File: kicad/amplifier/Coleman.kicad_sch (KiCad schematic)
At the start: 47 parts, among them Q1 TIP122, Q10 TIP122, Q11 IXTP6N50D2, Q12 BC550, Q13 BC550, Q14 TIP122, Q15 LND150, Q16 TIP122, Q17 BC550, Q19 LND150, Q2 TIP122, Q8 STP55NF06L

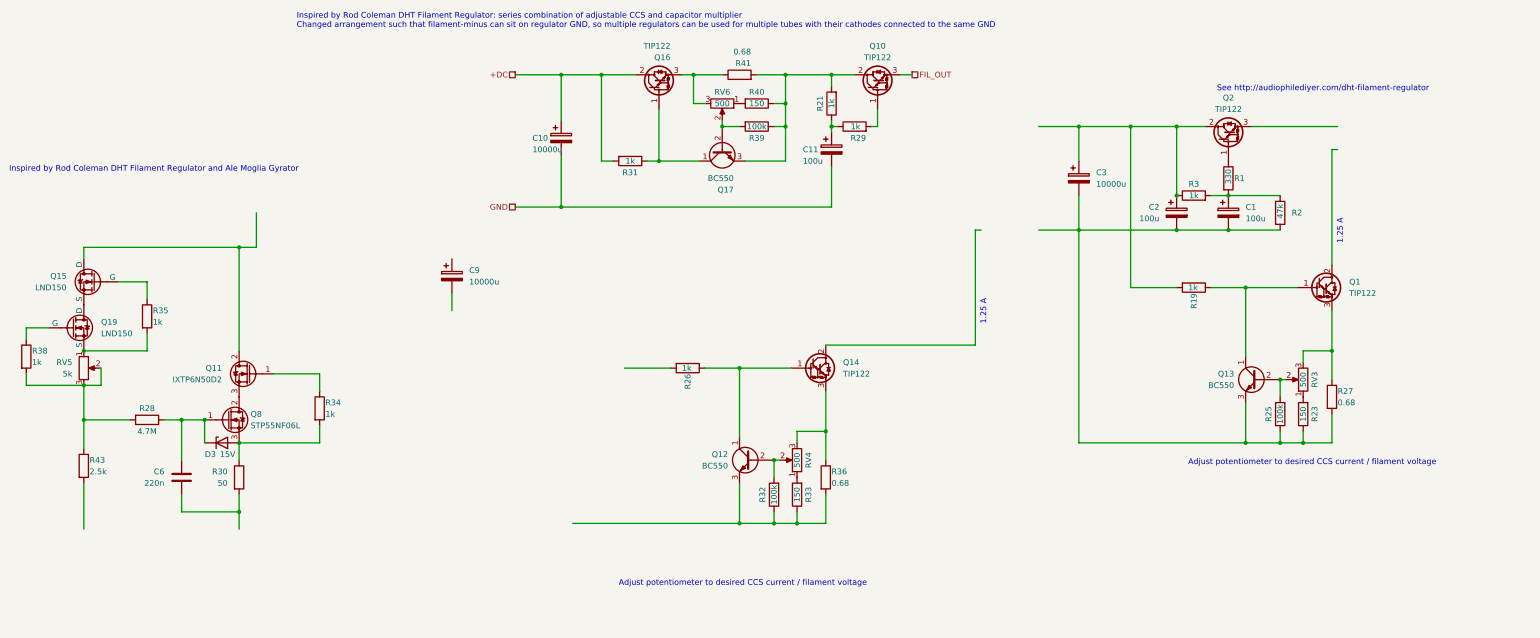
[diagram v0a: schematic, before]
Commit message: DHT fil reg
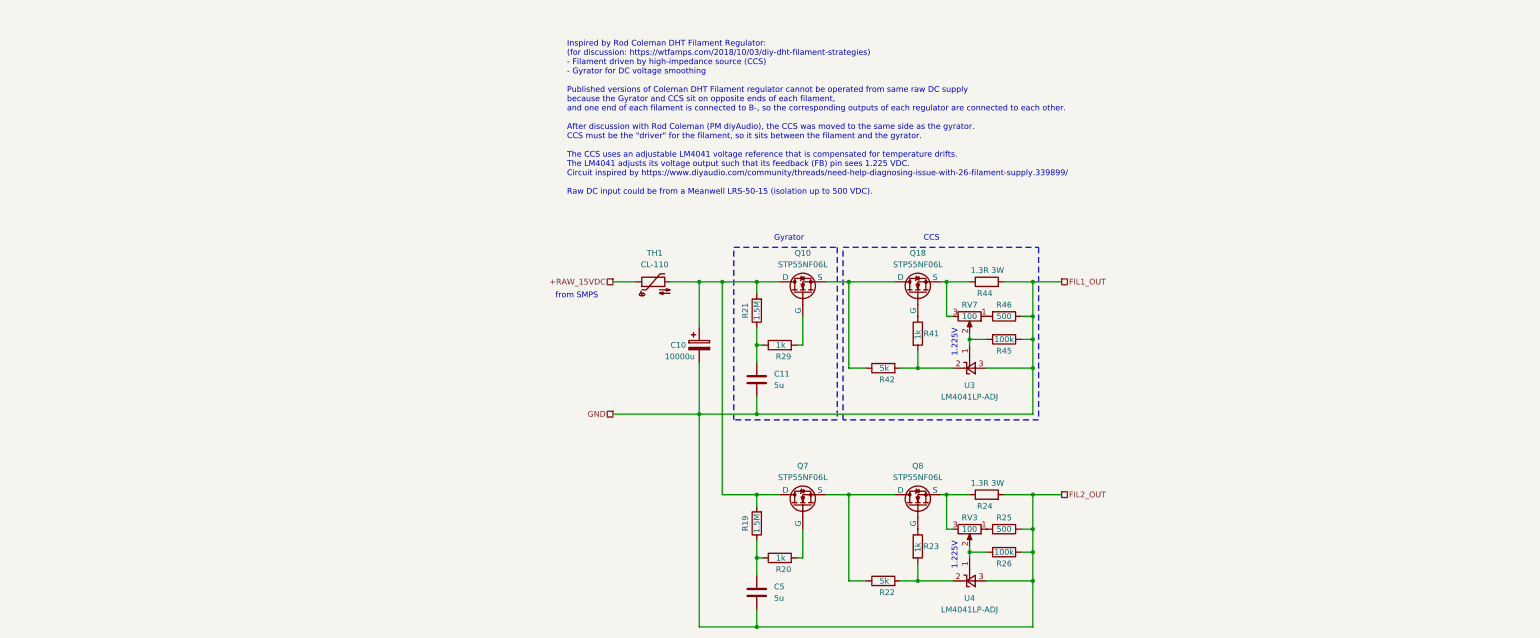
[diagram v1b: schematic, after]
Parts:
- removed C1, C11, C2: 100u, symbol Device:C_Polarized
- removed C3, C9: 10000u, Capacitor_THT:CP_Radial_D25.0mm_P10.00mm_SnapIn, symbol Device:C_Polarized
- removed C6: 220n, Capacitor_THT:C_Rect_L26.5mm_W10.5mm_P22.50mm_MKS4, symbol Device:C
- removed D3: 15V, Diode_THT:D_DO-34_SOD68_P7.62mm_Horizontal, symbol Device:D_Zener
- removed Q1, Q10, Q14, Q16, Q2: TIP122, Package_TO_SOT_THT:TO-220-3_Vertical, symbol Transistor_BJT:TIP122
- removed Q11: IXTP6N50D2, Package_TO_SOT_THT:TO-220-3_Vertical, symbol stax_ccs:10M90S
- removed Q12, Q13, Q17: BC550, Package_TO_SOT_THT:TO-92_Inline, symbol Transistor_BJT:BC550
- removed Q15, Q19: LND150, symbol Simulation_SPICE:NMOS
- removed Q8: STP55NF06L, Package_TO_SOT_THT:TO-220-3_Vertical, symbol Transistor_FET_Other:DN2540N5-G
- removed R1: 330, symbol Device:R
- removed R2: 47k, symbol Device:R
- removed R27, R36: 0.68, symbol Device:R
- removed R28: 4.7M, Resistor_THT:R_Axial_DIN0207_L6.3mm_D2.5mm_P10.16mm_Horizontal, symbol Device:R
- removed R3, R31: 1k, symbol Device:R
- removed R30: 50, Resistor_THT:R_Axial_DIN0207_L6.3mm_D2.5mm_P10.16mm_Horizontal, symbol Device:R
- removed R32, R39: 100k, symbol Device:R
- removed R33, R40: 150, symbol Device:R
- removed R34, R35, R38: 1k, Resistor_THT:R_Axial_DIN0207_L6.3mm_D2.5mm_P10.16mm_Horizontal, symbol Device:R
- removed R43: 2.5k, Resistor_THT:R_Axial_DIN0207_L6.3mm_D2.5mm_P10.16mm_Horizontal, symbol Device:R
- removed RV4, RV6: 500, symbol Device:R_Potentiometer
- removed RV5: 5k, symbol Device:R_Potentiometer
- added C11, C5: 5u, symbol Device:C
- added Q10, Q18, Q7, Q8: STP55NF06L, Package_TO_SOT_THT:TO-220-3_Vertical, symbol Simulation_SPICE:NMOS
- added R20: 1k, symbol Device:R
- added R22, R42: 5k, symbol Device:R
- added R24, R44: 1.3R 3W, Resistor_THT:R_Axial_DIN0617_L17.0mm_D6.0mm_P25.40mm_Horizontal, symbol Device:R
- added R45: 100k, symbol Device:R
- added R46: 500, symbol Device:R
- added RV7: 100, symbol Device:R_Potentiometer
- added TH1: CL-110, Varistor:RV_Disc_D12mm_W4.3mm_P7.5mm, symbol Device:Thermistor_NTC
- added U3, U4: LM4041LP-ADJ, Package_TO_SOT_THT:TO-92_Inline, symbol Reference_Voltage:LM4041LP-ADJ
- R19, R21: value 1k -> 1.5M
- R23: value 150 -> 1k
- R25: value 100k -> 500
- R26: value 1k -> 100k
- R41: value 0.68 -> 1k
- RV3: value 500 -> 100
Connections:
- net +DC is gone; now on an unnamed net: C10.1
- net GND is gone; now on net FIL1_OUT: C10.2
- net at R19.2: now also R21.2, Q10.1 (D), Q7.1 (D), TH1.2
- net at R23.1: now also Q8.2 (G); no longer R25.1
- net at R41.2: now also R42.2, U3.2 (K); no longer R21.2
- net FIL1_OUT: now reaches R26.1
- net FIL1_OUT: now also R25.1, C11.2, C5.2, R24.2, R44.2, R45.1, R46.1, U3.3 (A), U4.3 (A)
- net at R26.2: now also RV3.2, U4.1 (FB)
- net at R25.2: now also RV3.1; no longer RV3.2
- net at R41.1: now also Q18.2 (G)
- net at R21.1, R29.1: now also C11.1
- net at R29.2: now also Q10.2 (G)
- net at R19.1: now also C5.1, R20.1
- net at R23.2: now also R22.2, U4.2 (K); no longer RV3.1
- net at RV3.3: now also Q8.3 (S), R24.1
- new net: R45.2, RV7.2, U3.1 (FB)
- new net: Q10.3 (S), Q18.1 (D), R42.1
- new net: Q7.3 (S), Q8.1 (D), R22.1
- new net: Q18.3 (S), R44.1, RV7.3
- new net: Q7.2 (G), R20.2
- new net: R46.2, RV7.1
- new net +RAW_15VDC: TH1.1
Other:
- note added: "1.225V"
- note added: "CCS"
- note added: "Gyrator"
- note added: "Inspired by Rod Coleman DHT Filament Regulator: (for discussion: https://wtfamps.com/2018/10/03/diy-dht-filament-strategies) - Filament driven by high-impedance source (CCS) - Gyrator for DC voltage smoothing Published versions of Coleman DHT Filament regulator cannot be operated from same raw DC supply because the Gyrator and CCS sit on opposite ends of each filament, and one end of each filamen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"
- note added: "from SMPS"
- note removed: "1.25 A"
- note removed: "Adjust potentiometer to desired CCS current / filament voltage"
- note removed: "Inspired by Rod Coleman DHT Filament Regulator and Ale Moglia Gyrator"
- note removed: "Inspired by Rod Coleman DHT Filament Regulator: series combination of adjustable CCS and capacitor multiplier Changed arrangement such that filament-minus can sit on regulator GND, so multiple regulators can be used for multiple tubes with their cathodes connected to the same GND"
- note removed: "See http://audiophilediyer.com/dht-filament-regulator"
- moved on the sheet: C10, R21, R29
